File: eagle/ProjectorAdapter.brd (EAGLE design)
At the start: 18 x 35.5 mm, 9 parts, among them J1 05339805711, J2 05339805711, J3 0532610471

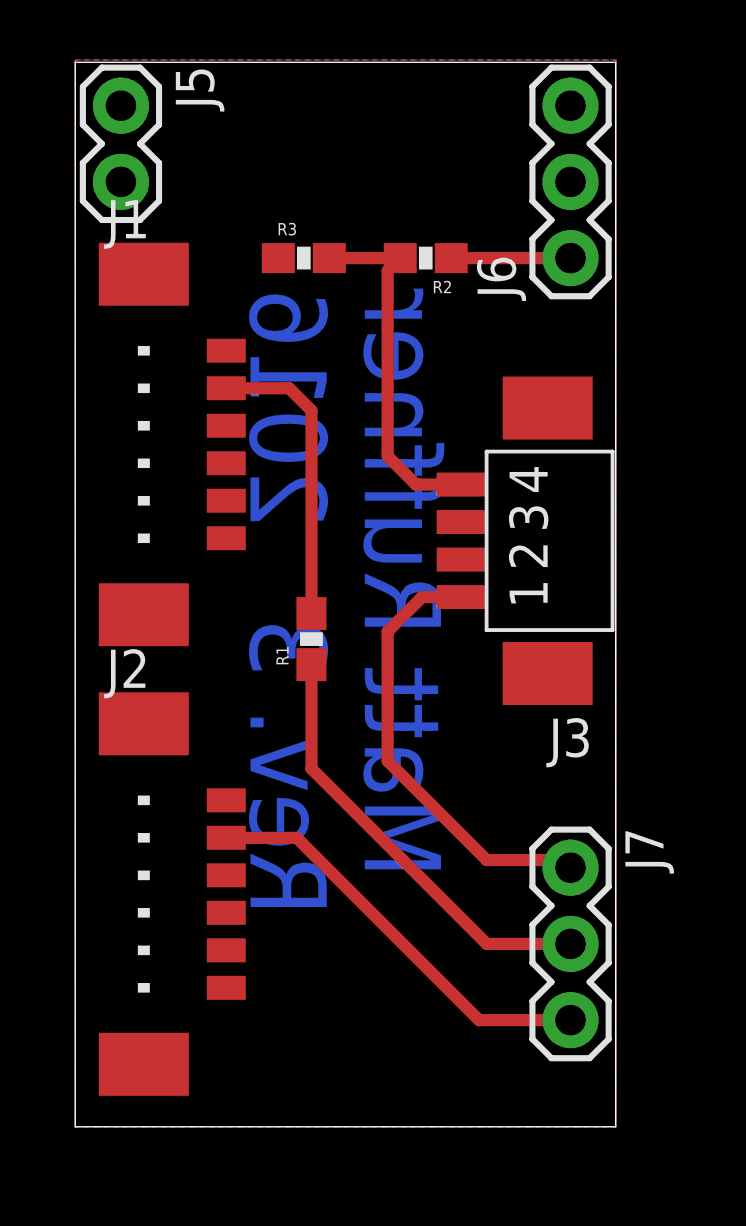
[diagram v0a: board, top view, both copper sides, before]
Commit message: added old silk changes
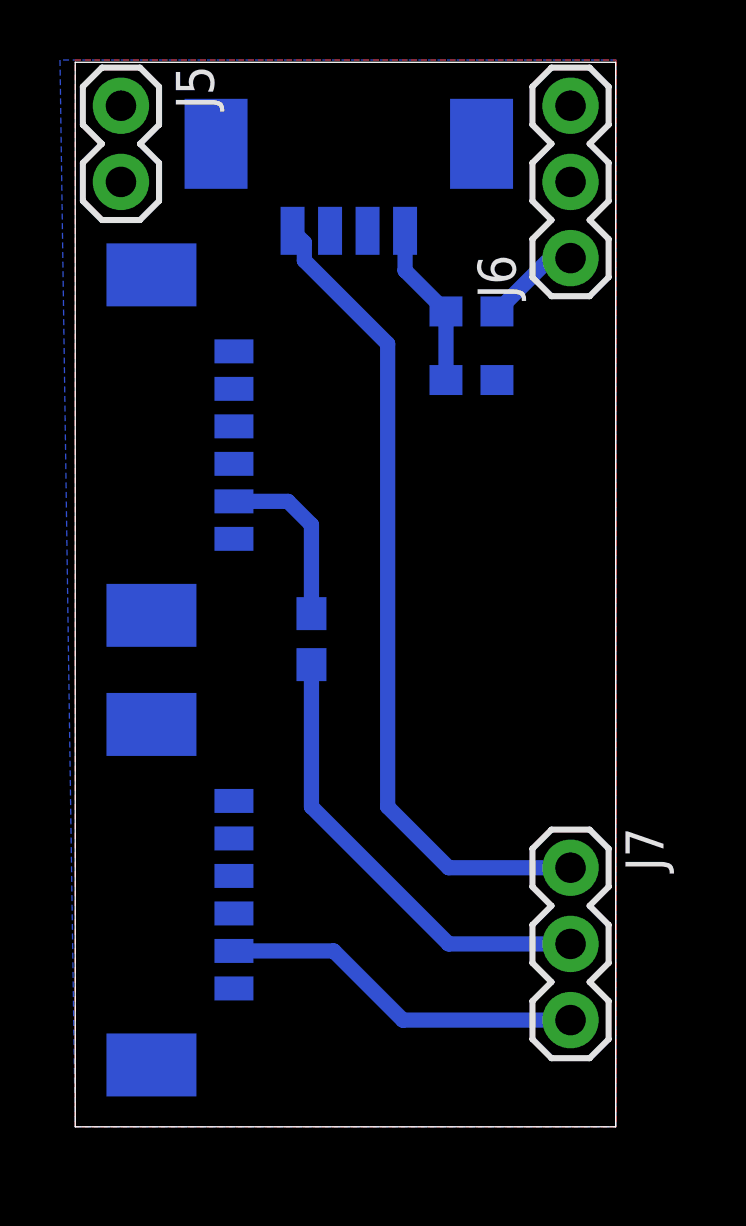
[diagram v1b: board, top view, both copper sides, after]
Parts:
- moved J3 14.8 mm to (9.14, 32.8), flipped to the bottom, turned to 180 degrees
- moved R3 6.91 mm to (13.2, 24.9), flipped to the bottom
- moved R2 2.34 mm to (13.2, 27.2), flipped to the bottom, turned to 0 degrees
- moved J1 1.30 mm to (2.54, 22.1), flipped to the bottom, turned to 90 degrees
- moved J2 1.30 mm to (2.54, 7.11), flipped to the bottom, turned to 90 degrees
- flipped R1 to the bottom
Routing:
- net TO_CAMERA: track 14.8 -> 27.8 mm
- net N$2: track 12.0 -> 5.54 mm
- net N$4: track 9.92 -> 5.87 mm
- net FROM_PROJ: track 14.0 -> 12.2 mm
- net 3V3: track 3.98 -> 3.19 mm
- net TO_PROJ: track 14.5 -> 15.3 mm
- added copper zone on layer 16, net GND
- removed copper zone on layer 16, net N$10
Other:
- board text removed: "Matt Ruffner Rev. 3 2016"
